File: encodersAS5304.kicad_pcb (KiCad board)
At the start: 2 copper layers, 11 parts, among them P1 CONN_01X02, P101 CONN_01X02, P102 CONN_01X02, P2 CONN_01X02, P3 CONN_01X02, P4 CONN_01X02, P5 CONN_01X02, P6 CONN_01X02, U101 AS5304

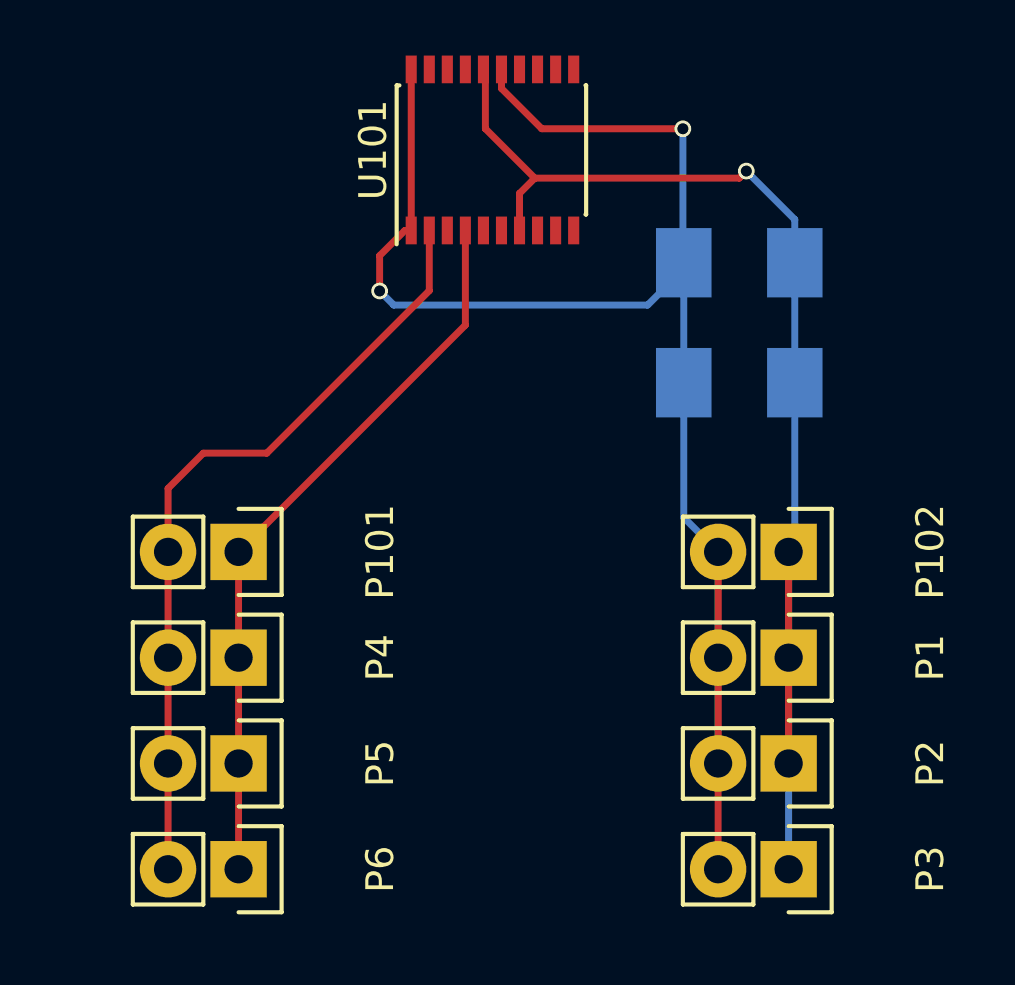
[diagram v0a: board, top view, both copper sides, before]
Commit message: placa con forma apropiada y dimensiones exactas. Falta enrutado
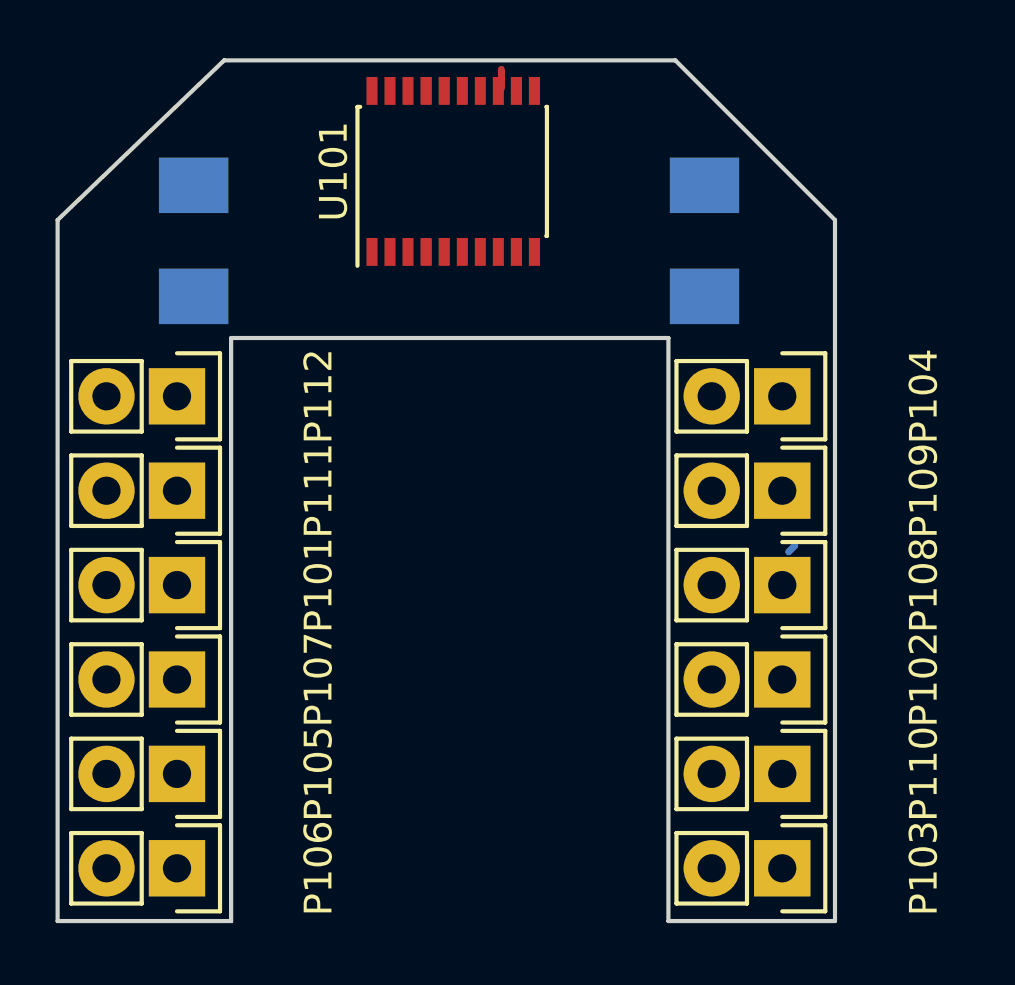
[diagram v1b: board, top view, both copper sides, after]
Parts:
- removed P1, P2, P3, P4, P5, P6: CONN_01X02, Pin_Headers:Pin_Header_Straight_1x02
- added P103: Pow, Pin_Headers:Pin_Header_Straight_1x02, F.Cu at (163.6, 119.6)
- added P104: Pow, Pin_Headers:Pin_Header_Straight_1x02, F.Cu at (163.6, 102.6)
- added P105: C1, Pin_Headers:Pin_Header_Straight_1x02, F.Cu at (141.8, 116.2)
- added P106: C1, Pin_Headers:Pin_Header_Straight_1x02, F.Cu at (141.8, 119.6)
- added P107: C1, Pin_Headers:Pin_Header_Straight_1x02, F.Cu at (141.8, 112.8)
- added P108: Pow, Pin_Headers:Pin_Header_Straight_1x02, F.Cu at (163.6, 109.4)
- added P109: Pow, Pin_Headers:Pin_Header_Straight_1x02, F.Cu at (163.6, 106.0)
- added P110: Pow, Pin_Headers:Pin_Header_Straight_1x02, F.Cu at (163.6, 116.2)
- added P111: C1, Pin_Headers:Pin_Header_Straight_1x02, F.Cu at (141.8, 106.0)
- added P112: C1, Pin_Headers:Pin_Header_Straight_1x02, F.Cu at (141.8, 102.6)
- P101: value CONN_01X02 -> C1
- P102: value CONN_01X02 -> Pow
- moved C101 19.7 mm to (142.4, 97.0), turned to 270 degrees
- moved C102 5.26 mm to (160.8, 97.0), turned to 270 degrees
- moved P102 4.60 mm to (163.6, 112.8)
- moved P101 2.52 mm to (141.8, 109.4)
- moved U101 1.61 mm to (151.8, 94.5)
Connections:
- U101 pad 10: Net-(U101-Pad10) -> (no net)
- U101 pad 11: Net-(U101-Pad11) -> (no net)
- U101 pad 12: Net-(U101-Pad12) -> (no net)
- U101 pad 13: Net-(U101-Pad13) -> (no net)
- U101 pad 14: Net-(U101-Pad14) -> (no net)
- U101 pad 17: Net-(U101-Pad17) -> (no net)
- U101 pad 18: Net-(U101-Pad18) -> (no net)
- U101 pad 19: Net-(U101-Pad19) -> (no net)
- U101 pad 5: Net-(U101-Pad5) -> (no net)
- U101 pad 6: Net-(U101-Pad6) -> (no net)
- U101 pad 8: Net-(U101-Pad8) -> (no net)
- U101 pad 9: Net-(U101-Pad9) -> (no net)
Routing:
- net GND: track 63.1 -> 0.00 mm, vias 2 -> 0
- net VDD: track 48.1 -> 0.00 mm, vias 1 -> 0
- net A: track 28.2 -> 0.00 mm
- net B: track 26.4 -> 0.00 mm
- net (no net): track 0.00 -> 1.00 mm
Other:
- board outline added: 28 x 31 mm
